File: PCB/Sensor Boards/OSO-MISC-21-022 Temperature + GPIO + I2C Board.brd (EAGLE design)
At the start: 14.4 x 6.6 mm, 9 parts

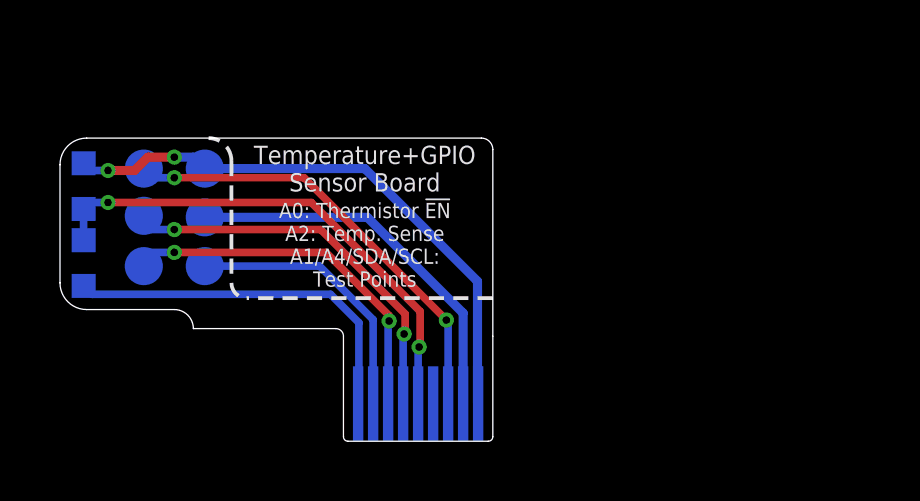
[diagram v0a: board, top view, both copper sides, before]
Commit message: more accelerometer and temperature board tests
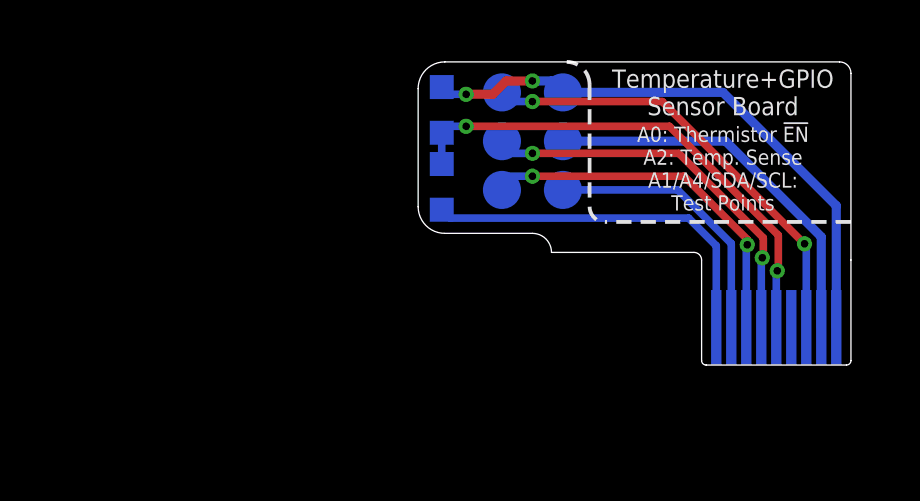
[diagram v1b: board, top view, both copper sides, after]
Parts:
- moved A4 12.2 mm to (2.79, 5.33)
- moved R1 12.2 mm to (0.79, 2.18)
- moved RT 12.2 mm to (0.79, 4.75)
- moved SDA 12.2 mm to (2.79, 2.08)
- moved U$3 12.2 mm to (11.9, -0.25)
- moved GND 12.2 mm to (4.83, 3.71)
- moved SCL 12.2 mm to (4.83, 2.08)
- moved VCC 12.2 mm to (4.83, 5.33)
- moved A1 12.2 mm to (2.79, 3.71)
